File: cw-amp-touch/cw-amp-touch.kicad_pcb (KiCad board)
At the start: 2 copper layers, 83 x 41 mm, 11 parts, among them J1 Conn_02x05_Odd_Even

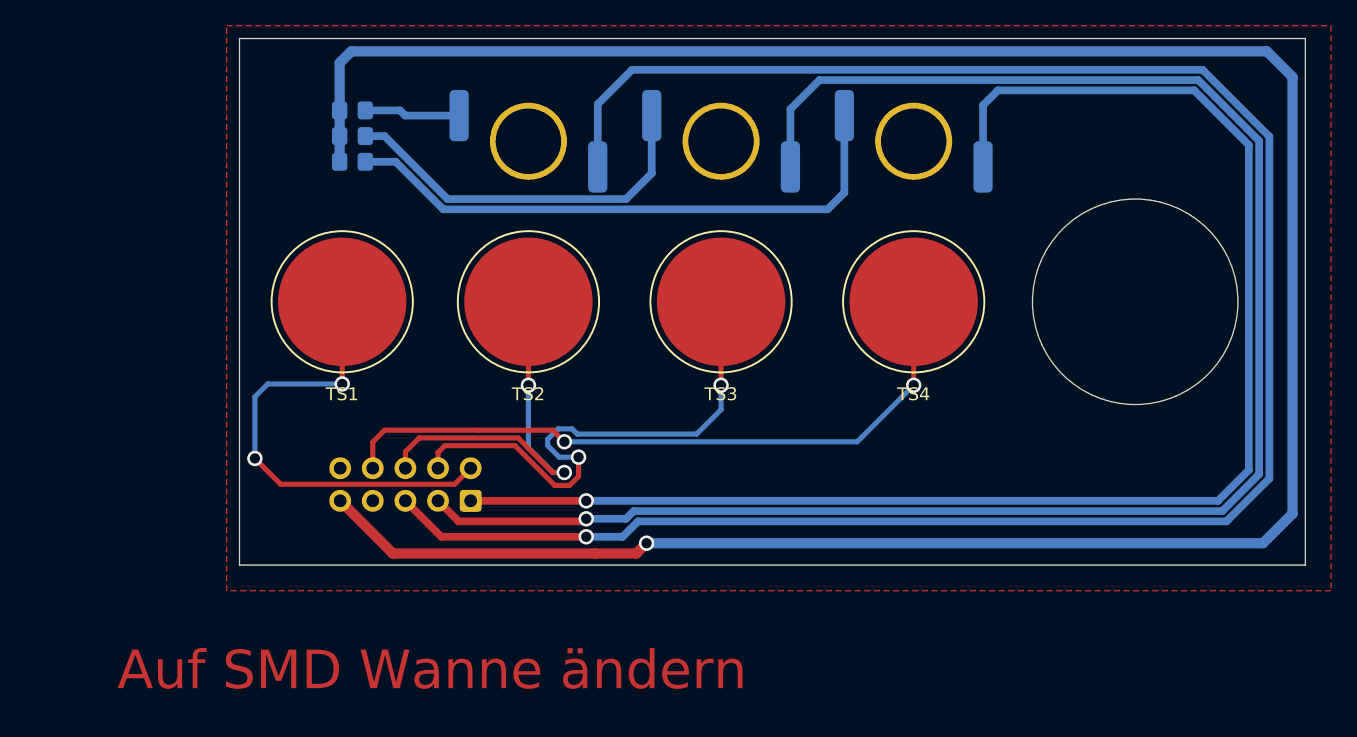
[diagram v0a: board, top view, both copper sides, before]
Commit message: tidy up folder structure
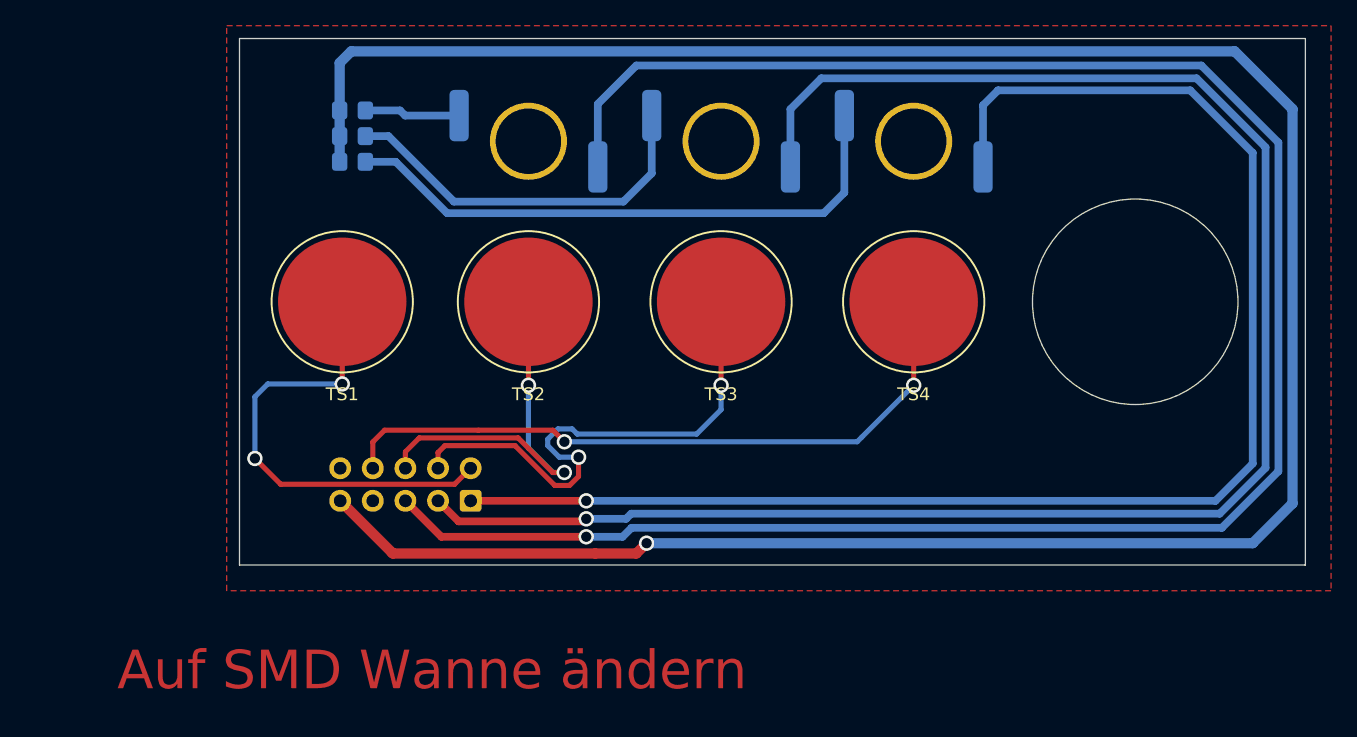
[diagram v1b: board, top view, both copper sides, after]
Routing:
- net +3V3: track 194.2 -> 192.3 mm
- net LED-ANALOG-INT: track 157.4 -> 158.5 mm
- net LED-ANALOG-EXT: track 136.0 -> 136.5 mm
